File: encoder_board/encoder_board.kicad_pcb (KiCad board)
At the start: 2 copper layers, 40 x 10 mm, 8 parts, among them J1 Conn_01x06, U1 AS5048A

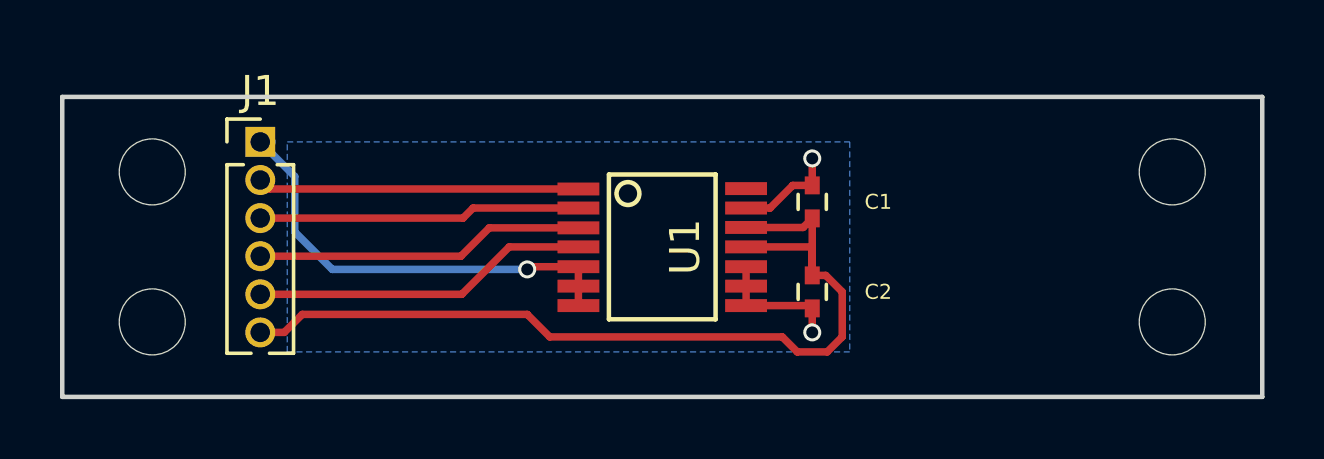
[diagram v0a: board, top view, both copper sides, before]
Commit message: reviewer final encoder board.
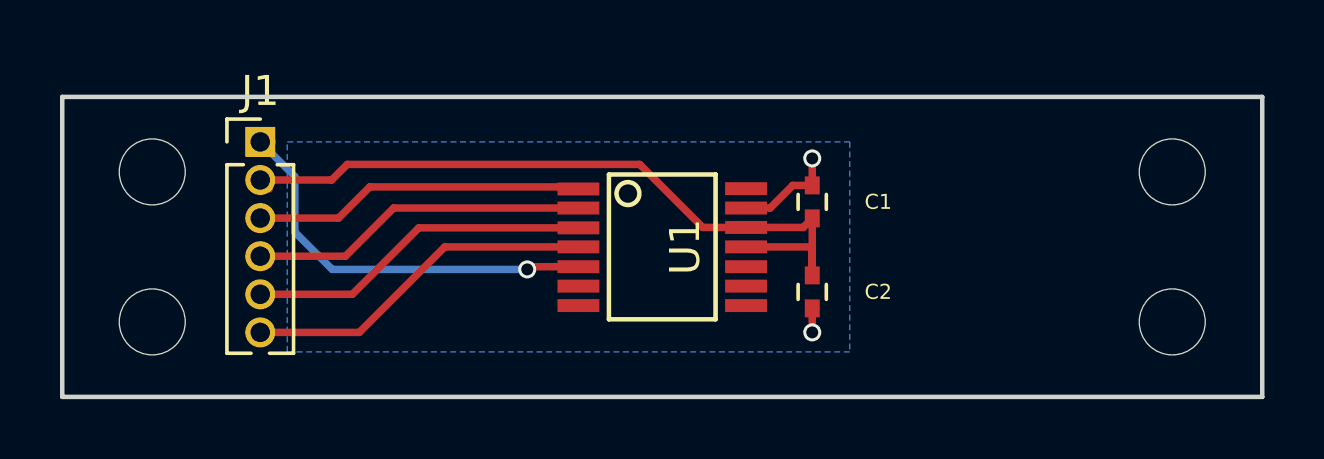
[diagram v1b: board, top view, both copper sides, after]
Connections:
- J1 pad 2: CS -> +3V3
- J1 pad 3: CLK -> CS
- J1 pad 4: MISO -> CLK
- J1 pad 5: MOSI -> MISO
- J1 pad 6: +3V3 -> MOSI
- U1 pad 10: GND -> Net-(U1-Pad10)
- U1 pad 6: GND -> Net-(U1-Pad6)
- U1 pad 7: GND -> Net-(U1-Pad7)
- U1 pad 8: GND -> Net-(U1-Pad8)
- U1 pad 9: GND -> Net-(U1-Pad9)
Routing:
- net +3V3: track 30.6 -> 25.1 mm
- net GND: track 22.9 -> 18.2 mm
- net MOSI: track 11.3 -> 11.8 mm
- net CLK: track 10.7 -> 11.3 mm
- net MISO: track 11.0 -> 11.5 mm
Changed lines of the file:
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@@
 (kicad_pcb (version 4) (host pcbnew 4.0.7-e2-6376~58~ubuntu16.04.1)
   (general
-    (links 17)
+    (links 12)
     (no_connects 0)
-    (area 92.942857 98.325 146.057143 112.575)
+    (area 99.924999 99.924999 140.075001 110.075001)
     (thickness 1.6)
     (drawings 6)
-    (tracks 49)
+    (tracks 40)
     (zones 0)
     (modules 8)
-    (nets 8)
+    (nets 13)
   )
   (page A4)
@@
   (net 6 MISO)
   (net 7 MOSI)
+  (net 8 "Net-(U1-Pad6)")
+  (net 9 "Net-(U1-Pad7)")
+  (net 10 "Net-(U1-Pad8)")
+  (net 11 "Net-(U1-Pad9)")
+  (net 12 "Net-(U1-Pad10)")
   (net_class Default "This is the default net class."
     (clearance 0.2)
@@
     (add_net MISO)
     (add_net MOSI)
+    (add_net "Net-(U1-Pad10)")
     (add_net "Net-(U1-Pad14)")
+    (add_net "Net-(U1-Pad6)")
+    (add_net "Net-(U1-Pad7)")
+    (add_net "Net-(U1-Pad8)")
+    (add_net "Net-(U1-Pad9)")
   )
   (module Mounting_Holes:MountingHole_2.2mm_M2 (layer F.Cu)
@@
       (net 1 GND))
     (pad 6 smd rect (at 1.3081 2.794 270) (size 0.4318 1.397) (layers F.Cu F.Paste F.Mask)
-      (net 1 GND))
+      (net 8 "Net-(U1-Pad6)"))
     (pad 7 smd rect (at 1.9558 2.794 270) (size 0.4318 1.397) (layers F.Cu F.Paste F.Mask)
-      (net 1 GND))
+      (net 9 "Net-(U1-Pad7)"))
     (pad 8 smd rect (at 1.9558 -2.794 270) (size 0.4318 1.397) (layers F.Cu F.Paste F.Mask)
-      (net 1 GND))
+      (net 10 "Net-(U1-Pad8)"))
     (pad 9 smd rect (at 1.3081 -2.794 270) (size 0.4318 1.397) (layers F.Cu F.Paste F.Mask)
-      (net 1 GND))
+      (net 11 "Net-(U1-Pad9)"))
     (pad 10 smd rect (at 0.6604 -2.794 270) (size 0.4318 1.397) (layers F.Cu F.Paste F.Mask)
-      (net 1 GND))
+      (net 12 "Net-(U1-Pad10)"))
     (pad 11 smd rect (at 0 -2.794 270) (size 0.4318 1.397) (layers F.Cu F.Paste F.Mask)
       (net 3 +3V3))
@@
       (net 1 GND))
     (pad 2 thru_hole oval (at 0 1.27) (size 1 1) (drill 0.65) (layers *.Cu *.Mask)
+      (net 3 +3V3))
+    (pad 3 thru_hole oval (at 0 2.54) (size 1 1) (drill 0.65) (layers *.Cu *.Mask)
       (net 4 CS))
-    (pad 3 thru_hole oval (at 0 2.54) (size 1 1) (drill 0.65) (layers *.Cu *.Mask)
+    (pad 4 thru_hole oval (at 0 3.81) (size 1 1) (drill 0.65) (layers *.Cu *.Mask)
       (net 5 CLK))
-    (pad 4 thru_hole oval (at 0 3.81) (size 1 1) (drill 0.65) (layers *.Cu *.Mask)
+    (pad 5 thru_hole oval (at 0 5.08) (size 1 1) (drill 0.65) (layers *.Cu *.Mask)
       (net 6 MISO))
-    (pad 5 thru_hole oval (at 0 5.08) (size 1 1) (drill 0.65) (layers *.Cu *.Mask)
+    (pad 6 thru_hole oval (at 0 6.35) (size 1 1) (drill 0.65) (layers *.Cu *.Mask)
       (net 7 MOSI))
-    (pad 6 thru_hole oval (at 0 6.35) (size 1 1) (drill 0.65) (layers *.Cu *.Mask)
-      (net 3 +3V3))
     (model Pin_Headers.3dshapes/Pin_Header_Straight_1x06_Pitch1.27mm.wrl
       (at (xyz 0 0 0))
@@
   (segment (start 125 107.05) (end 125 107.85) (width 0.25) (layer F.Cu) (net 1))
   (via (at 125 107.85) (size 0.6) (drill 0.4) (layers F.Cu B.Cu) (net 1))
-  (segment (start 122.794 106.9558) (end 124.9058 106.9558) (width 0.25) (layer F.Cu) (net 1))
   (segment (start 124.9058 106.9558) (end 125 107.05) (width 0.25) (layer F.Cu) (net 1))
   (segment (start 125 102.95) (end 125 102.05) (width 0.25) (layer F.Cu) (net 1))
@@
   (segment (start 124.35 102.95) (end 125 102.95) (width 0.25) (layer F.Cu) (net 1))
   (segment (start 123.5954 103.7046) (end 124.35 102.95) (width 0.25) (layer F.Cu) (net 1))
-  (segment (start 122.794 106.3081) (end 122.794 105.6604) (width 0.25) (layer F.Cu) (net 1))
-  (segment (start 122.794 106.9558) (end 122.794 106.3081) (width 0.25) (layer F.Cu) (net 1))
-  (segment (start 117.206 106.3081) (end 117.206 105.6604) (width 0.25) (layer F.Cu) (net 1))
-  (segment (start 117.206 106.9558) (end 117.206 106.3081) (width 0.25) (layer F.Cu) (net 1))
+  (segment (start 121.3523 104.3523) (end 122.794 104.3523) (width 0.25) (layer F.Cu) (net 3))
+  (segment (start 119.25 102.25) (end 121.3523 104.3523) (width 0.25) (layer F.Cu) (net 3))
+  (segment (start 109.5 102.25) (end 119.25 102.25) (width 0.25) (layer F.Cu) (net 3))
+  (segment (start 108.98 102.77) (end 109.5 102.25) (width 0.25) (layer F.Cu) (net 3))
+  (segment (start 106.6 102.77) (end 108.98 102.77) (width 0.25) (layer F.Cu) (net 3))
   (segment (start 122.794 104.3523) (end 124.6977 104.3523) (width 0.25) (layer F.Cu) (net 3))
   (segment (start 124.6977 104.3523) (end 125 104.05) (width 0.25) (layer F.Cu) (net 3))
-  (segment (start 106.6 107.85) (end 107.4 107.85) (width 0.25) (layer F.Cu) (net 3))
-  (segment (start 125.45 105.95) (end 125 105.95) (width 0.25) (layer F.Cu) (net 3))
-  (segment (start 126 106.5) (end 125.45 105.95) (width 0.25) (layer F.Cu) (net 3))
-  (segment (start 126 108) (end 126 106.5) (width 0.25) (layer F.Cu) (net 3))
-  (segment (start 125.5 108.5) (end 126 108) (width 0.25) (layer F.Cu) (net 3))
-  (segment (start 124.5 108.5) (end 125.5 108.5) (width 0.25) (layer F.Cu) (net 3))
-  (segment (start 124 108) (end 124.5 108.5) (width 0.25) (layer F.Cu) (net 3))
-  (segment (start 116.25 108) (end 124 108) (width 0.25) (layer F.Cu) (net 3))
-  (segment (start 115.5 107.25) (end 116.25 108) (width 0.25) (layer F.Cu) (net 3))
-  (segment (start 108 107.25) (end 115.5 107.25) (width 0.25) (layer F.Cu) (net 3))
-  (segment (start 107.4 107.85) (end 108 107.25) (width 0.25) (layer F.Cu) (net 3))
   (segment (start 125 105.95) (end 125 105) (width 0.25) (layer F.Cu) (net 3))
   (segment (start 125 105) (end 122.794 105) (width 0.25) (layer F.Cu) (net 3))
-  (segment (start 106.65 107.9) (end 106.6 107.85) (width 0.25) (layer F.Cu) (net 3))
   (segment (start 125 105.95) (end 125 104.05) (width 0.25) (layer F.Cu) (net 3))
-  (segment (start 117.206 103.0696) (end 106.8996 103.0696) (width 0.25) (layer F.Cu) (net 4) (status 20))
-  (segment (start 106.8996 103.0696) (end 106.6 102.77) (width 0.25) (layer F.Cu) (net 4) (status 30))
-  (segment (start 106.6 104.04) (end 113.36 104.04) (width 0.25) (layer F.Cu) (net 5) (status 10))
-  (segment (start 113.36 104.04) (end 113.6954 103.7046) (width 0.25) (layer F.Cu) (net 5))
-  (segment (start 113.6954 103.7046) (end 117.206 103.7046) (width 0.25) (layer F.Cu) (net 5))
-  (segment (start 106.6 105.31) (end 113.29 105.31) (width 0.25) (layer F.Cu) (net 6) (status 10))
-  (segment (start 113.29 105.31) (end 114.235 104.365) (width 0.25) (layer F.Cu) (net 6))
-  (segment (start 114.235 104.365) (end 117.206 104.365) (width 0.25) (layer F.Cu) (net 6))
-  (segment (start 106.6 106.58) (end 113.32 106.58) (width 0.25) (layer F.Cu) (net 7) (status 10))
-  (segment (start 113.32 106.58) (end 114.9 105) (width 0.25) (layer F.Cu) (net 7))
-  (segment (start 114.9 105) (end 117.206 105) (width 0.25) (layer F.Cu) (net 7))
+  (segment (start 106.8996 103.0696) (end 106.6 102.77) (width 0.25) (layer F.Cu) (net 3) (status 30))
+  (segment (start 106.6 104.04) (end 109.21 104.04) (width 0.25) (layer F.Cu) (net 4))
+  (segment (start 110.25 103) (end 117.1364 103) (width 0.25) (layer F.Cu) (net 4))
+  (segment (start 109.21 104.04) (end 110.25 103) (width 0.25) (layer F.Cu) (net 4))
+  (segment (start 117.1364 103) (end 117.206 103.0696) (width 0.25) (layer F.Cu) (net 4))
+  (segment (start 106.6 105.31) (end 109.44 105.31) (width 0.25) (layer F.Cu) (net 5))
+  (segment (start 111.0454 103.7046) (end 117.206 103.7046) (width 0.25) (layer F.Cu) (net 5))
+  (segment (start 109.44 105.31) (end 111.0454 103.7046) (width 0.25) (layer F.Cu) (net 5))
+  (segment (start 106.6 106.58) (end 109.67 106.58) (width 0.25) (layer F.Cu) (net 6))
+  (segment (start 111.885 104.365) (end 117.206 104.365) (width 0.25) (layer F.Cu) (net 6))
+  (segment (start 109.67 106.58) (end 111.885 104.365) (width 0.25) (layer F.Cu) (net 6))
+  (segment (start 106.6 107.85) (end 109.9 107.85) (width 0.25) (layer F.Cu) (net 7))
+  (segment (start 112.75 105) (end 117.206 105) (width 0.25) (layer F.Cu) (net 7))
+  (segment (start 109.9 107.85) (end 112.75 105) (width 0.25) (layer F.Cu) (net 7))
   (zone (net 1) (net_name GND) (layer B.Cu) (hatch edge 0.508)
     (connect_pads (clearance 0.25))
